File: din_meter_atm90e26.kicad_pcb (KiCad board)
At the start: 2 copper layers, 29 x 31.2 mm, 60 parts, among them J1 USEL, J2 MMD1, J3 MMD0, J4 CONN_02X18, J5 CONN_01X10, J6 USEL, J7 MMD1, J8 MMD0, M1 ATM90E26_ATM90E26, M2 ATM90E26_ATM90E26, Y1 Crystal_Small, Y2 Crystal_Small

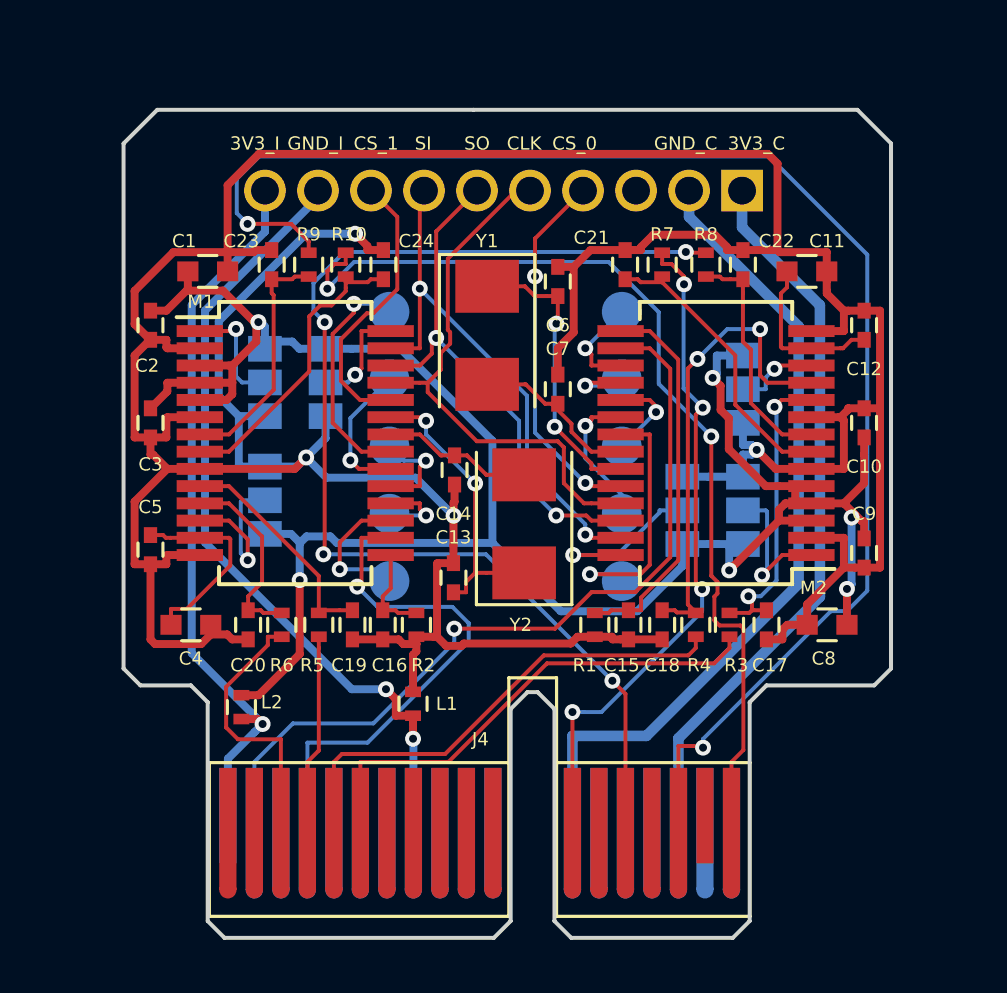
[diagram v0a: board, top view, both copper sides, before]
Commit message: Rerouted board from joslyn
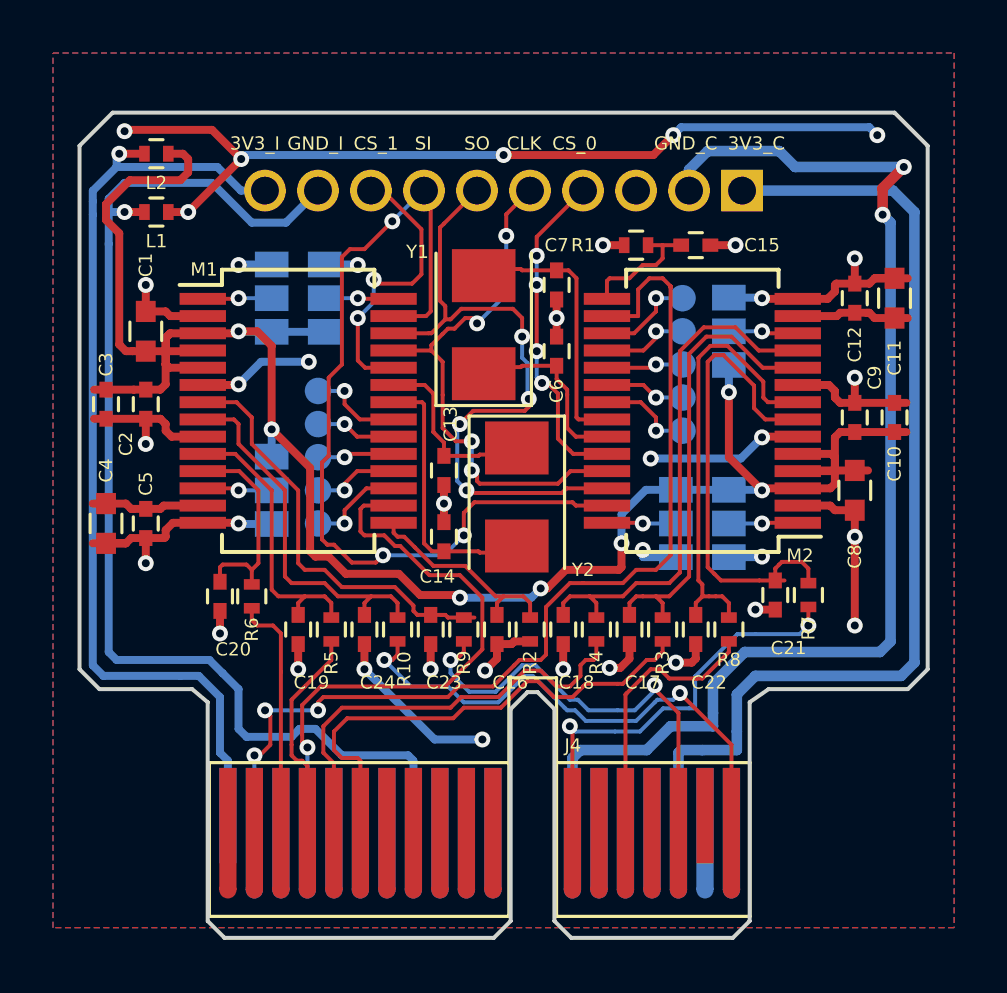
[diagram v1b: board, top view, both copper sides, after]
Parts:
- removed G1: LOGO, Whatnick_logo:Whatnick_logo
- removed LOGO1: Logo_Open_Hardware_Small, Symbols:OSHW-Logo2_7.3x6mm_SilkScreen
- moved L2 21.1 mm to (132.8, 60.0), turned to 0 degrees
- moved L1 20.9 mm to (132.8, 62.1), turned to 0 degrees
- moved C23 15.0 mm to (143.2, 77.9), turned to 90 degrees
- moved R9 15.0 mm to (144.4, 77.9), turned to 270 degrees
- moved C15 14.5 mm to (153.2, 63.4), turned to 180 degrees
- moved R1 14.4 mm to (150.9, 63.4), turned to 180 degrees
- moved R10 13.9 mm to (141.9, 77.9), turned to 270 degrees
- moved C22 13.9 mm to (153.2, 77.9), turned to 90 degrees
- moved R8 13.8 mm to (154.4, 77.9), turned to 270 degrees
- moved C24 13.8 mm to (140.7, 77.9), turned to 90 degrees
- moved C21 13.7 mm to (156.2, 76.6), turned to 90 degrees
- moved R7 13.6 mm to (157.4, 76.6), turned to 270 degrees
- moved ZX_0 6.12 mm to (152.7, 70.4)
- moved C8 5.18 mm to (159.2, 72.7), turned to 270 degrees
- moved C17 5.17 mm to (150.7, 77.9)
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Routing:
- net GNDD: track 165.3 -> 108.0 mm, vias 4 -> 37
- net I2P_1_IN: track 56.2 -> 16.9 mm
- net I2N_0_IN: track 44.4 -> 10.3 mm, vias 4 -> 0
- net I2N_1_IN: track 37.2 -> 20.4 mm
- net GND_ISO: track 30.2 -> 44.6 mm, vias 2 -> 1
- net GND_CPU: track 31.0 -> 45.2 mm, vias 0 -> 2
- net SI/RX: track 20.4 -> 34.2 mm, vias 2 -> 3
- net 3V3_CPU: track 27.5 -> 38.3 mm
- net VN_0: track 14.4 -> 4.88 mm
- net I2P_0_IN: track 25.5 -> 16.0 mm, vias 4 -> 2
- net 3V3_ISO: track 27.3 -> 36.5 mm
- net I2N_0: track 9.01 -> 16.7 mm
- net I2P_0: track 11.0 -> 18.3 mm
- net I2P_1: track 9.12 -> 15.9 mm
- net VP_0: track 31.0 -> 37.8 mm, vias 1 -> 3
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- added copper zone on B.Cu, net GNDD
- added copper zone on F.Cu, net GNDD
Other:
- board size 29 x 31.2 mm -> 32 x 31.1 mm
- rule pad_to_mask_clearance: 0.2 -> 0.15
